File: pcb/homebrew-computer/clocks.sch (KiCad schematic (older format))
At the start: 11 parts, among them J5 Conn_01x04_Male, J6 Conn_01x02, U16 DS1077LZ-60+, U17 74LVC1G157GC-Q100H, U18 74LVC1G14GW,125

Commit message: Keep working on the layout
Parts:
- J5: footprint Connector_PinHeader_2.54mm:PinHeader_2x02_P2.54mm_Vertical -> Connector_Molex:Molex_Pico-Clasp_202396-0607_1x06-1MP_P1.00mm_Horizontal
- J6: footprint Connector_Molex:Molex_PicoBlade_53048-0210_1x02_P1.25mm_Horizontal -> Connector_Molex:Molex_Pico-Clasp_202396-0207_1x02-1MP_P1.00mm_Horizontal
- R7: footprint Resistor_SMD:R_0603_1608Metric -> Resistor_SMD:R_0402_1005Metric_Pad0.72x0.64mm_HandSolder
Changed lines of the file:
@@
 F 0 "J5" H 3272 1282 50  0000 R CNN
 F 1 "Conn_01x04_Male" H 3650 1050 50  0000 R CNN
-F 2 "Connector_PinHeader_2.54mm:PinHeader_2x02_P2.54mm_Vertical" H 3300 1400 50  0001 C CNN
+F 2 "Connector_Molex:Molex_Pico-Clasp_202396-0607_1x06-1MP_P1.00mm_Horizontal" H 3300 1400 50  0001 C CNN
 F 3 "~" H 3300 1400 50  0001 C CNN
 	1    3300 1400
@@
 F 0 "R7" H 1209 3396 50  0000 L CNN
 F 1 "10k" H 1209 3305 50  0000 L CNN
-F 2 "Resistor_SMD:R_0603_1608Metric" H 1150 3350 50  0001 C CNN
+F 2 "Resistor_SMD:R_0402_1005Metric_Pad0.72x0.64mm_HandSolder" H 1150 3350 50  0001 C CNN
 F 3 "~" H 1150 3350 50  0001 C CNN
 	1    1150 3350
@@
 F 0 "J6" H 3250 3400 50  0000 L CNN
 F 1 "Conn_01x02" H 3000 3300 50  0000 L CNN
-F 2 "Connector_Molex:Molex_PicoBlade_53048-0210_1x02_P1.25mm_Horizontal" H 3450 3150 50  0001 C CNN
+F 2 "Connector_Molex:Molex_Pico-Clasp_202396-0207_1x02-1MP_P1.00mm_Horizontal" H 3450 3150 50  0001 C CNN
 F 3 "~" H 3450 3150 50  0001 C CNN
 	1    3450 3150

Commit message: Add the board outline
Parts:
- U17: footprint Package_SO:TSOP-6_1.65x3.05mm_P0.95mm -> Package_TO_SOT_SMD:SOT-363_SC-70-6_Handsoldering
- U18: footprint Package_SO:TSSOP-5 -> Package_TO_SOT_SMD:SOT-353_SC-70-5_Handsoldering
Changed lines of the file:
@@
 F 0 "U17" H 5137 2065 50  0000 C CNN
 F 1 "74LVC1G157GC-Q100H" H 4950 2000 50  0000 C CNN
-F 2 "Package_SO:TSOP-6_1.65x3.05mm_P0.95mm" H 5150 2000 50  0001 C CNN
+F 2 "Package_TO_SOT_SMD:SOT-363_SC-70-6_Handsoldering" H 5150 2000 50  0001 C CNN
 F 3 "" H 5150 2000 50  0001 C CNN
 	1    5150 2000
@@
 F 0 "U18" H 7775 2115 50  0000 C CNN
 F 1 "74LVC1G14GW,125" H 7775 2024 50  0000 C CNN
-F 2 "Package_SO:TSSOP-5" H 7800 2050 50  0001 C CNN
+F 2 "Package_TO_SOT_SMD:SOT-353_SC-70-5_Handsoldering" H 7800 2050 50  0001 C CNN
 F 3 "" H 7800 2050 50  0001 C CNN
 	1    7800 2050

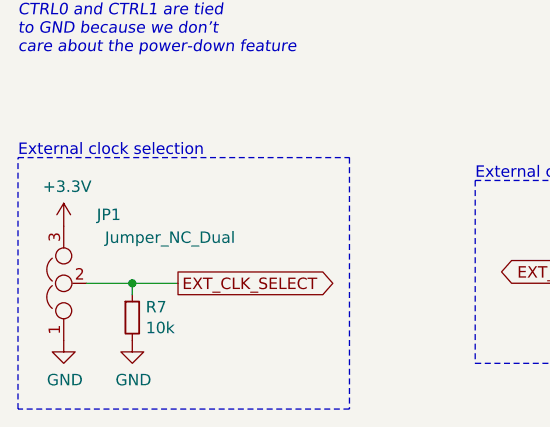
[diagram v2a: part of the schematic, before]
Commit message: Keep working on the layout
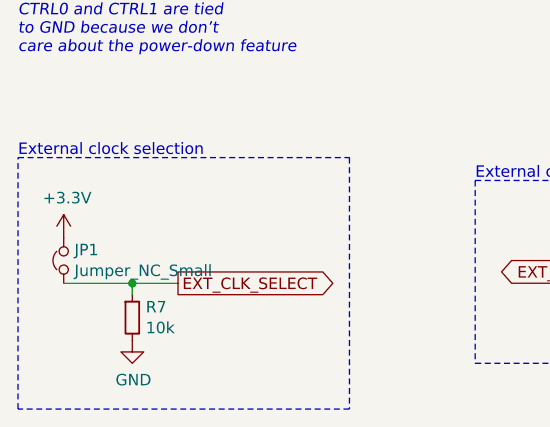
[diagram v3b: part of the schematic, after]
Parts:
- removed JP1: Jumper_NC_Dual, Jumper:SolderJumper-3_P1.3mm_Open_RoundedPad1.0x1.5mm, symbol Device:Jumper_NC_Dual
- added JP1: Jumper_NC_Small, Jumper:SolderJumper-2_P1.3mm_Open_RoundedPad1.0x1.5mm, symbol Device:Jumper_NC_Small
- J5: footprint Connector_Molex:Molex_Pico-Clasp_202396-0607_1x06-1MP_P1.00mm_Horizontal -> Connector_Molex:Molex_Pico-Clasp_202396-0407_1x04-1MP_P1.00mm_Horizontal
- U17: footprint Package_TO_SOT_SMD:SOT-363_SC-70-6_Handsoldering -> Package_TO_SOT_SMD:SOT-363_SC-70-6
- U18: footprint Package_TO_SOT_SMD:SOT-353_SC-70-5_Handsoldering -> Package_TO_SOT_SMD:SOT-353_SC-70-5
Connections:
- net +3V3: now also JP1.2
- net EXT_CLK_SELECT: now also JP1.1
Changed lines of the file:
@@
 F 0 "J5" H 3272 1282 50  0000 R CNN
 F 1 "Conn_01x04_Male" H 3650 1050 50  0000 R CNN
-F 2 "Connector_Molex:Molex_Pico-Clasp_202396-0607_1x06-1MP_P1.00mm_Horizontal" H 3300 1400 50  0001 C CNN
+F 2 "Connector_Molex:Molex_Pico-Clasp_202396-0407_1x04-1MP_P1.00mm_Horizontal" H 3300 1400 50  0001 C CNN
 F 3 "~" H 3300 1400 50  0001 C CNN
 	1    3300 1400
@@
 Clock inversion
 $Comp
-L Device:Jumper_NC_Dual JP1
-U 1 1 5FB84D34
-P 850 3200
-F 0 "JP1" V 1150 2950 50  0000 L CNN
-F 1 "Jumper_NC_Dual" V 1050 2450 50  0000 L CNN
-F 2 "Jumper:SolderJumper-3_P1.3mm_Open_RoundedPad1.0x1.5mm" H 850 3200 50  0001 C CNN
-F 3 "~" H 850 3200 50  0001 C CNN
-	1    850  3200
-	0    -1   -1   0
-$EndComp
-$Comp
-L power:GND #PWR0146
-U 1 1 5FB8AE54
-P 850 3450
-F 0 "#PWR0146" H 850 3200 50  0001 C CNN
-F 1 "GND" H 855 3277 50  0000 C CNN
-F 2 "" H 850 3450 50  0001 C CNN
-F 3 "" H 850 3450 50  0001 C CNN
-	1    850  3450
-	1    0    0    -1
-$EndComp
-$Comp
 L power:+3.3V #PWR0147
 U 1 1 5FB8B254
-P 850 2950
-F 0 "#PWR0147" H 850 2800 50  0001 C CNN
-F 1 "+3.3V" H 865 3123 50  0000 C CNN
-F 2 "" H 850 2950 50  0001 C CNN
-F 3 "" H 850 2950 50  0001 C CNN
-	1    850  2950
+P 850 3000
+F 0 "#PWR0147" H 850 2850 50  0001 C CNN
+F 1 "+3.3V" H 865 3173 50  0000 C CNN
+F 2 "" H 850 3000 50  0001 C CNN
+F 3 "" H 850 3000 50  0001 C CNN
+	1    850  3000
 	1    0    0    -1
 $EndComp
@@
 	1    0    0    -1
 $EndComp
-Wire Wire Line
-	950  3200 1150 3200
 $Comp
 L power:GND #PWR0148
@@
 F 0 "U17" H 5137 2065 50  0000 C CNN
 F 1 "74LVC1G157GC-Q100H" H 4950 2000 50  0000 C CNN
-F 2 "Package_TO_SOT_SMD:SOT-363_SC-70-6_Handsoldering" H 5150 2000 50  0001 C CNN
+F 2 "Package_TO_SOT_SMD:SOT-363_SC-70-6" H 5150 2000 50  0001 C CNN
 F 3 "" H 5150 2000 50  0001 C CNN
 	1    5150 2000
@@
 F 0 "U18" H 7775 2115 50  0000 C CNN
 F 1 "74LVC1G14GW,125" H 7775 2024 50  0000 C CNN
-F 2 "Package_TO_SOT_SMD:SOT-353_SC-70-5_Handsoldering" H 7800 2050 50  0001 C CNN
+F 2 "Package_TO_SOT_SMD:SOT-353_SC-70-5" H 7800 2050 50  0001 C CNN
 F 3 "" H 7800 2050 50  0001 C CNN
 	1    7800 2050
 	1    0    0    -1
 $EndComp
+$Comp
+L Device:Jumper_NC_Small JP1
+U 1 1 5FAADF33
+P 850 3100
+F 0 "JP1" V 896 3053 50  0000 R CNN
+F 1 "Jumper_NC_Small" V 805 3053 50  0000 R CNN
+F 2 "Jumper:SolderJumper-2_P1.3mm_Open_RoundedPad1.0x1.5mm" H 850 3100 50  0001 C CNN
+F 3 "~" H 850 3100 50  0001 C CNN
+	1    850  3100
+	0    -1   -1   0
+$EndComp
+Wire Wire Line
+	850  3200 1150 3200
 $EndSCHEMATC
